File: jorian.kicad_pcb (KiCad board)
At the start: 2 copper layers, 99.1 x 99.7 mm, 107 parts, among them J1 MicroUSB, J2 USB-C, J3 MicroUSB, J4 USB-C, J5 MJ-4PP-9, SW1 SW_SPDT, U3 AMS1117, U4 TP4056, U5 DW01A, U6 FS8205A

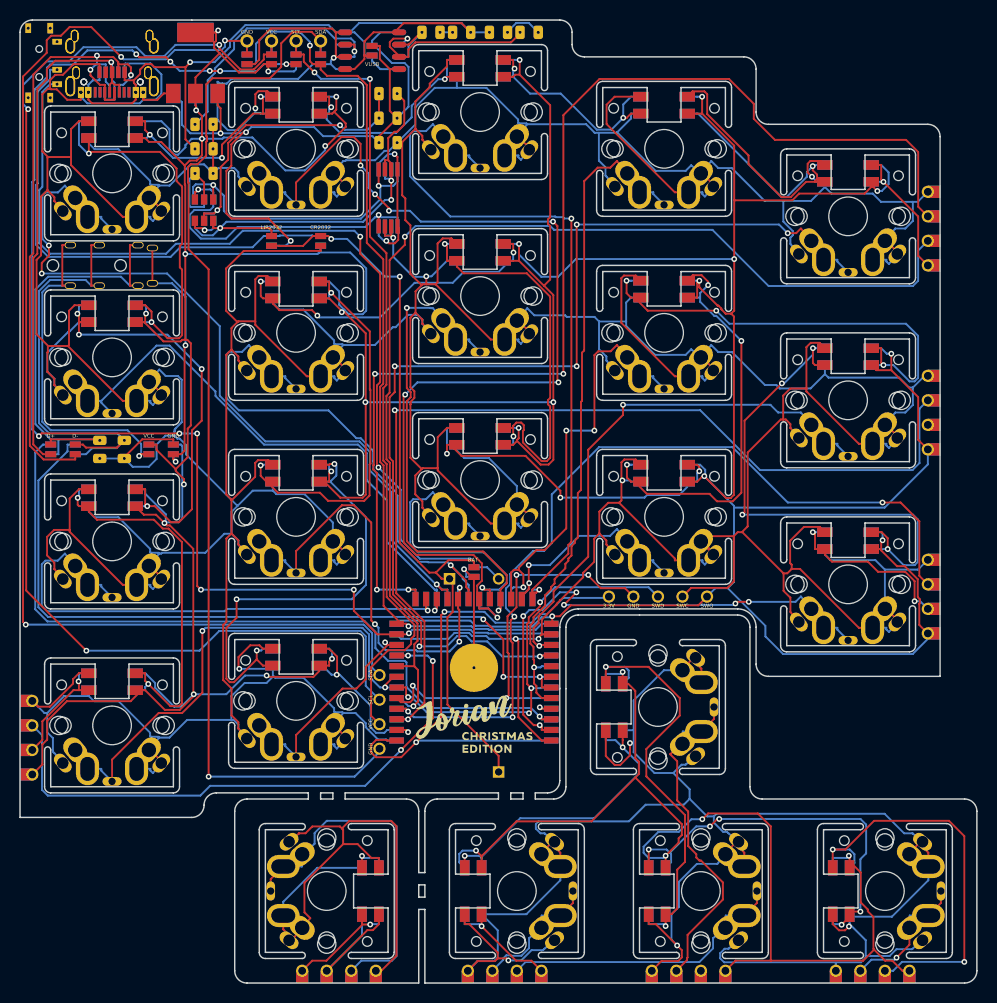
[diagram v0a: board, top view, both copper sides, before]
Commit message: updated placement
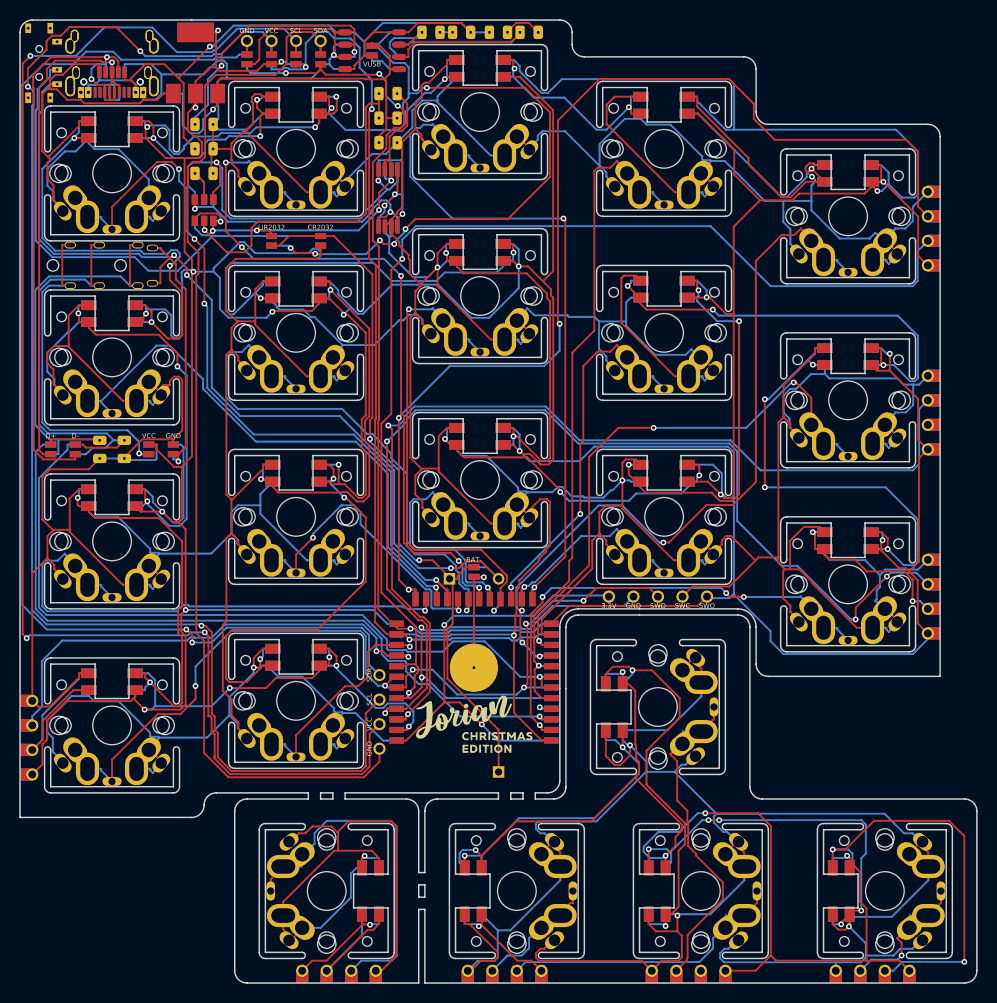
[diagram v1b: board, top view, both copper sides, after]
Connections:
- J4 pad A6: D+ -> Net-(J4-PadA6)
- J4 pad A7: D- -> Net-(J4-PadA7)
- J4 pad B6: D+ -> Net-(J4-PadA6)
- J4 pad B7: D- -> Net-(J4-PadA7)
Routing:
- net VCC: track 608.3 -> 683.9 mm, vias 28 -> 23
- net Net-(JP4-Pad2): track 84.2 -> 149.1 mm, vias 2 -> 3
- net SCL: track 139.5 -> 94.7 mm, vias 11 -> 3
- net LIPO+: track 76.6 -> 113.3 mm, vias 3 -> 7
- net /S2: track 110.6 -> 77.9 mm, vias 7 -> 5
- net /S5: track 111.5 -> 79.8 mm, vias 6 -> 4
- net /S21: track 91.5 -> 109.7 mm
- net Net-(JP3-Pad2): track 131.8 -> 145.8 mm
- net /S12: track 47.7 -> 35.2 mm, vias 3 -> 2
- net /S18: track 63.5 -> 51.3 mm, vias 3 -> 2
- net Net-(L7-Pad1): track 36.0 -> 48.0 mm, vias 3 -> 2
- net SWO: track 56.6 -> 45.6 mm
- net /S19: track 126.2 -> 116.5 mm, vias 4 -> 3
- net /DIN18: track 13.6 -> 21.8 mm, vias 1 -> 0
- net Net-(U5-Pad1): track 32.2 -> 40.3 mm
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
